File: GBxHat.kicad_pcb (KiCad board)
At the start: 2 copper layers, 65 x 30 mm, 26 parts, among them IC1 ATMEGA8515L-8AU, J0 Pi Zero, J1 AVR_SPI_6, U1 TXB0108PWR, U2 NLAS4157, X1 8MHz

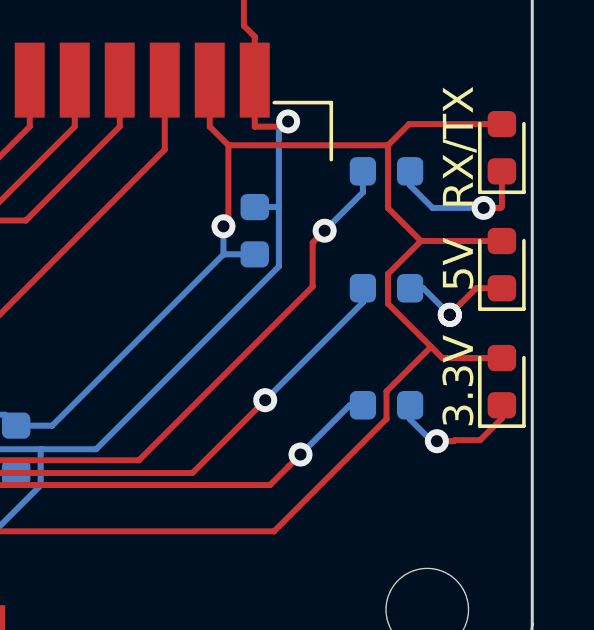
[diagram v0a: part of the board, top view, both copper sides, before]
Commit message: small update
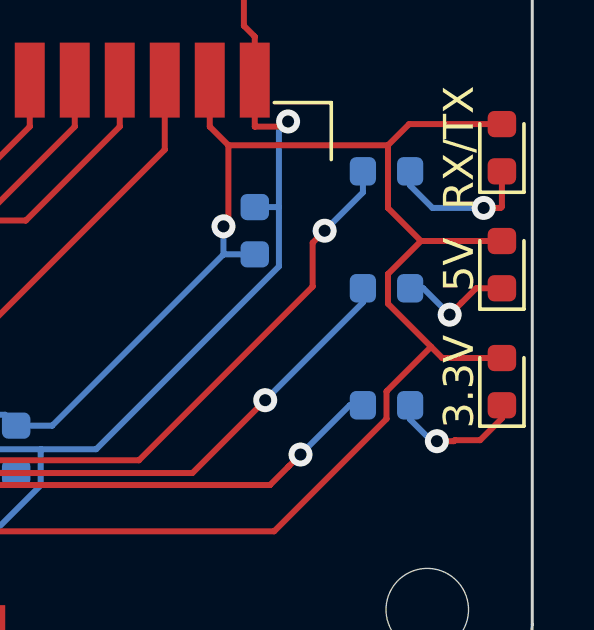
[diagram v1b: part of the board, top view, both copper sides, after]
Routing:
- net Net-(LED2-Pad1): vias 2 -> 1
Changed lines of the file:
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@@
     (thickness 1.6)
     (drawings 10)
-    (tracks 729)
+    (tracks 728)
     (zones 0)
     (modules 26)
@@
   (segment (start 261.1935 83.0382) (end 261.631 83.0382) (width 0.2) (layer B.Cu) (net 58))
   (segment (start 262.51043 83.91763) (end 262.52202 83.92922) (width 0.2) (layer B.Cu) (net 58))
-  (via (at 262.51043 83.91763) (size 0.8) (drill 0.4) (layers F.Cu B.Cu) (net 58))
   (segment (start 262.52202 83.92922) (end 262.52202 83.92922) (width 0.2) (layer B.Cu) (net 58))
-  (via (at 262.52202 83.92922) (size 0.8) (drill 0.4) (layers F.Cu B.Cu) (net 58))
   (segment (start 262.910429 83.517631) (end 262.51043 83.91763) (width 0.2) (layer F.Cu) (net 58))
   (segment (start 263.38986 83.0382) (end 262.910429 83.517631) (width 0.2) (layer F.Cu) (net 58))
   (segment (start 264.252 83.0382) (end 263.38986 83.0382) (width 0.2) (layer F.Cu) (net 58))
+  (via (at 262.51043 83.91763) (size 0.8) (drill 0.4) (layers F.Cu B.Cu) (net 58) (status 1000000))
   (segment (start 261.1935 79.6157) (end 261.93832 80.36052) (width 0.2) (layer B.Cu) (net 59))
   (segment (start 261.1935 79.1407) (end 261.1935 79.6157) (width 0.2) (layer B.Cu) (net 59))
